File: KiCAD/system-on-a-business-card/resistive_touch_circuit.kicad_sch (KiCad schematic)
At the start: 21 parts, among them U5 TCA9535PWR

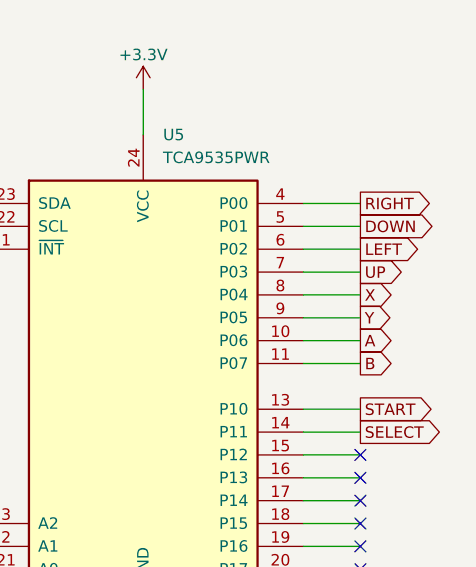
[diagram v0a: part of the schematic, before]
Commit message: #10: started with routing
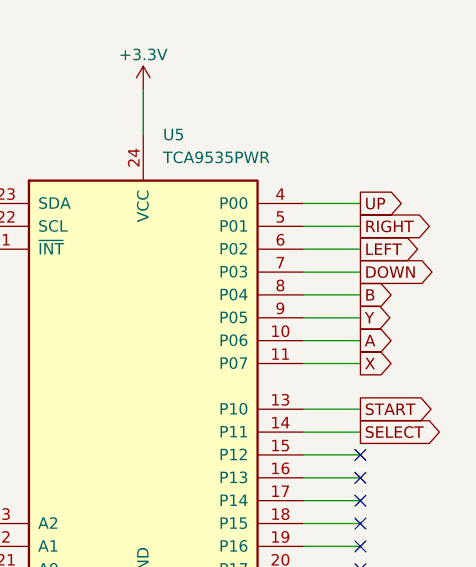
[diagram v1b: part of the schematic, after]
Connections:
- net B: now also U5.8 (P04); no longer U5.11 (P07)
- net DOWN: now also U5.7 (P03); no longer U5.5 (P01)
- net RIGHT: now also U5.5 (P01); no longer U5.4 (P00)
- net UP: now also U5.4 (P00); no longer U5.7 (P03)
- net X: now also U5.11 (P07); no longer U5.8 (P04)
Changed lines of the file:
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@@
     )
   )
-  (global_label "X" (shape output) (at 195.58 55.88 0) (fields_autoplaced)
+  (global_label "X" (shape output) (at 195.58 63.5 0) (fields_autoplaced)
     (effects (font (size 1.27 1.27)) (justify left))
-    (property "Intersheetrefs" "${INTERSHEET_REFS}" (at 199.7747 55.88 0)
+    (property "Intersheetrefs" "${INTERSHEET_REFS}" (at 199.7747 63.5 0)
       (effects (font (size 1.27 1.27)) (justify left) hide)
     )
@@
     )
   )
-  (global_label "B" (shape output) (at 195.58 63.5 0) (fields_autoplaced)
+  (global_label "B" (shape output) (at 195.58 55.88 0) (fields_autoplaced)
     (effects (font (size 1.27 1.27)) (justify left))
-    (property "Intersheetrefs" "${INTERSHEET_REFS}" (at 199.8352 63.5 0)
+    (property "Intersheetrefs" "${INTERSHEET_REFS}" (at 199.8352 55.88 0)
       (effects (font (size 1.27 1.27)) (justify left) hide)
     )
@@
     )
   )
-  (global_label "UP" (shape output) (at 195.58 53.34 0) (fields_autoplaced)
+  (global_label "UP" (shape output) (at 195.58 45.72 0) (fields_autoplaced)
     (effects (font (size 1.27 1.27)) (justify left))
-    (property "Intersheetrefs" "${INTERSHEET_REFS}" (at 201.1657 53.34 0)
+    (property "Intersheetrefs" "${INTERSHEET_REFS}" (at 201.1657 45.72 0)
       (effects (font (size 1.27 1.27)) (justify left) hide)
     )
@@
     )
   )
-  (global_label "DOWN" (shape output) (at 195.58 48.26 0) (fields_autoplaced)
+  (global_label "DOWN" (shape output) (at 195.58 53.34 0) (fields_autoplaced)
     (effects (font (size 1.27 1.27)) (justify left))
-    (property "Intersheetrefs" "${INTERSHEET_REFS}" (at 203.9476 48.26 0)
+    (property "Intersheetrefs" "${INTERSHEET_REFS}" (at 203.9476 53.34 0)
       (effects (font (size 1.27 1.27)) (justify left) hide)
     )
   )
-  (global_label "RIGHT" (shape output) (at 195.58 45.72 0) (fields_autoplaced)
+  (global_label "RIGHT" (shape output) (at 195.58 48.26 0) (fields_autoplaced)
     (effects (font (size 1.27 1.27)) (justify left))
-    (property "Intersheetrefs" "${INTERSHEET_REFS}" (at 204.0081 45.72 0)
+    (property "Intersheetrefs" "${INTERSHEET_REFS}" (at 204.0081 48.26 0)
       (effects (font (size 1.27 1.27)) (justify left) hide)
     )

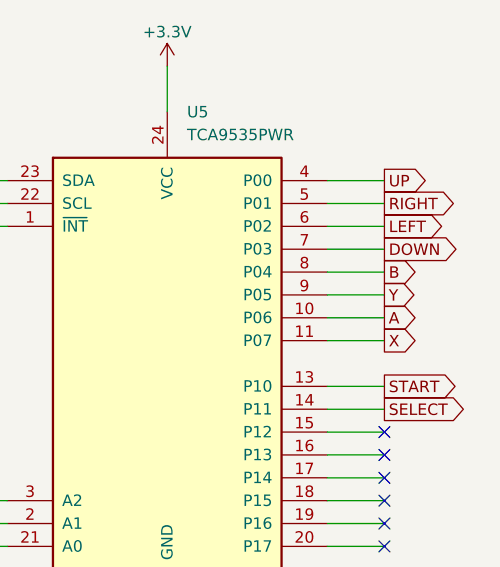
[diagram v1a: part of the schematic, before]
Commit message: #10: continued with routing
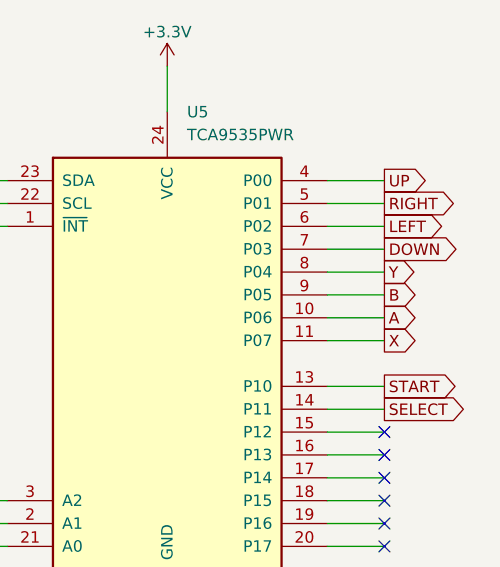
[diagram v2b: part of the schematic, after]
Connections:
- net B: now also U5.9 (P05); no longer U5.8 (P04)
- net Y: now also U5.8 (P04); no longer U5.9 (P05)
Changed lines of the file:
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@@
     )
   )
-  (global_label "B" (shape output) (at 195.58 55.88 0) (fields_autoplaced)
+  (global_label "B" (shape output) (at 195.58 58.42 0) (fields_autoplaced)
     (effects (font (size 1.27 1.27)) (justify left))
-    (property "Intersheetrefs" "${INTERSHEET_REFS}" (at 199.8352 55.88 0)
+    (property "Intersheetrefs" "${INTERSHEET_REFS}" (at 199.8352 58.42 0)
       (effects (font (size 1.27 1.27)) (justify left) hide)
     )
@@
     )
   )
-  (global_label "Y" (shape output) (at 195.58 58.42 0) (fields_autoplaced)
+  (global_label "Y" (shape output) (at 195.58 55.88 0) (fields_autoplaced)
     (effects (font (size 1.27 1.27)) (justify left))
-    (property "Intersheetrefs" "${INTERSHEET_REFS}" (at 199.6538 58.42 0)
+    (property "Intersheetrefs" "${INTERSHEET_REFS}" (at 199.6538 55.88 0)
       (effects (font (size 1.27 1.27)) (justify left) hide)
     )
